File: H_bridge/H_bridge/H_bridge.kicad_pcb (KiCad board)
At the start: 2 copper layers, 49.8 x 36 mm, 19 parts, among them J1 Screw_Terminal_01x02, J2 Screw_Terminal_01x06, J3 Pins_02x10_P1.27mm_TH, U1 VNH7040AYTR

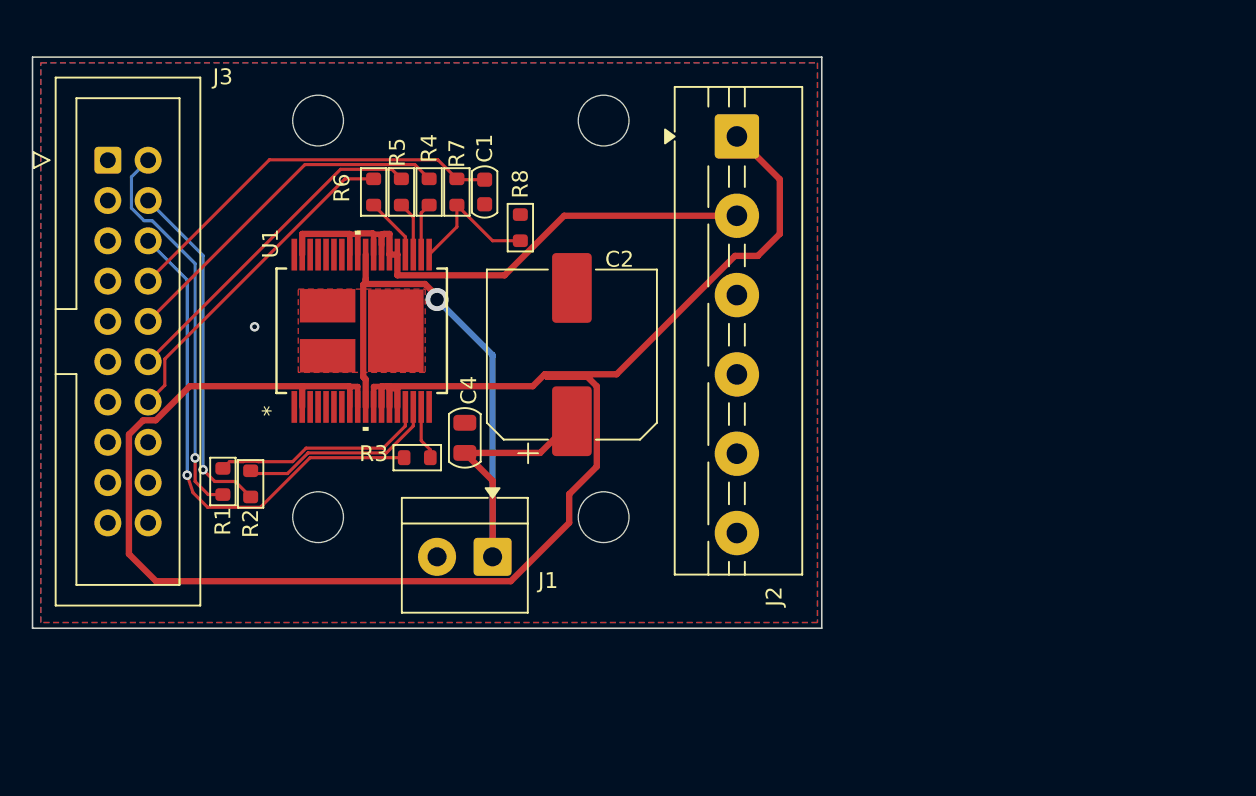
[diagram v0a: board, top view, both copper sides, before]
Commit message: avances pcb
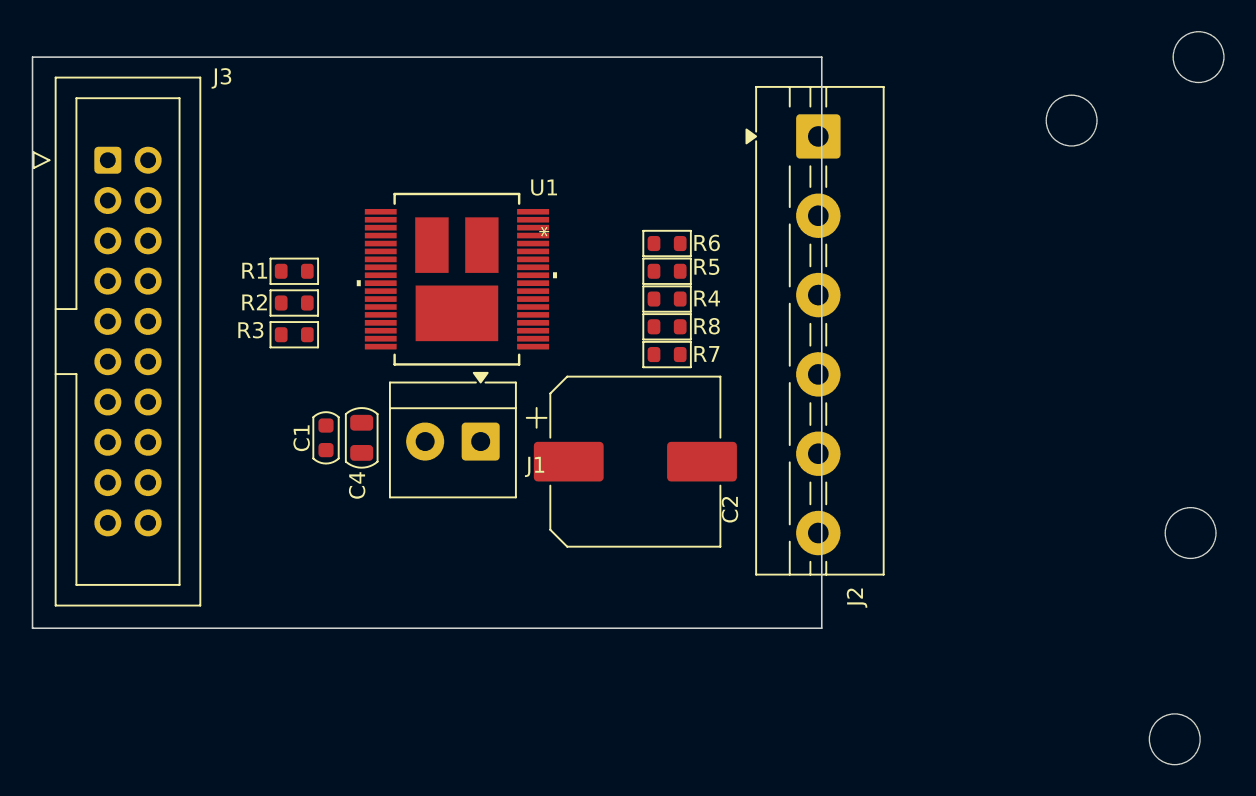
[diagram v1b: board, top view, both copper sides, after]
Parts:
- moved H1 55.8 mm to (184.2, 92.8)
- moved H4 55.6 mm to (185.8, 49.8)
- moved H3 37.0 mm to (185.2, 79.8)
- moved H2 29.5 mm to (177.8, 53.8)
- moved R6 18.8 mm to (152.2, 61.5), turned to 180 degrees
- moved C1 18.4 mm to (130.8, 73.8)
- moved R5 17.5 mm to (152.2, 63.2), turned to 180 degrees
- moved R7 16.8 mm to (152.2, 68.5), turned to 180 degrees
- moved R4 16.4 mm to (152.2, 65.0), turned to 180 degrees
- moved R1 14.0 mm to (128.8, 63.2), turned to 0 degrees
- moved R2 11.7 mm to (128.8, 65.2), turned to 0 degrees
- moved R8 11.2 mm to (152.2, 66.8), turned to 180 degrees
- moved R3 11.0 mm to (128.8, 67.2)
- moved C2 7.85 mm to (150.2, 75.2), turned to 0 degrees
- moved J1 7.31 mm to (140.5, 74.0)
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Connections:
- U1 pad 37: Heatsink -> +24V
- U1 pad 38: Heatsink -> /Drain_Low_SideA
- U1 pad 39: Heatsink -> /Drain_Low_SideB
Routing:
- net /Drain_Low_SideA: track 113.7 -> 0.00 mm
- net +24V: track 47.3 -> 0.00 mm, vias 1 -> 0
- net /Drain_Low_SideB: track 38.1 -> 0.00 mm
- net Net-(J3-Pad6): track 31.9 -> 0.00 mm, vias 1 -> 0
- net Net-(C1-Pad1): track 24.9 -> 0.00 mm
- net Net-(J3-Pad2): track 24.7 -> 0.00 mm, vias 1 -> 0
- net Net-(J3-Pad10): track 22.2 -> 0.00 mm
- net Net-(J3-Pad4): track 22.1 -> 0.00 mm, vias 1 -> 0
- net Net-(J3-Pad14): track 21.8 -> 0.00 mm
- net Net-(J3-Pad12): track 21.2 -> 0.00 mm
- net /SEL0: track 13.8 -> 0.00 mm
- net /INA: track 12.8 -> 0.00 mm
- net /CS/DF: track 8.78 -> 0.00 mm
- net /SEL1: track 3.95 -> 0.00 mm
- net /PWM: track 3.44 -> 0.00 mm
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- removed copper zone on B.Cu, net GND
- removed copper zone on F.Cu, net GND
- removed copper zone on F.Cu, net Heatsink
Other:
- copper layers 2 -> 4
